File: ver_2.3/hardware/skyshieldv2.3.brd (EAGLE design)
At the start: 17.8 x 43.2 mm, 11 parts, among them J1 HEAD15-NOSS, J2 HEAD15-NOSS-1

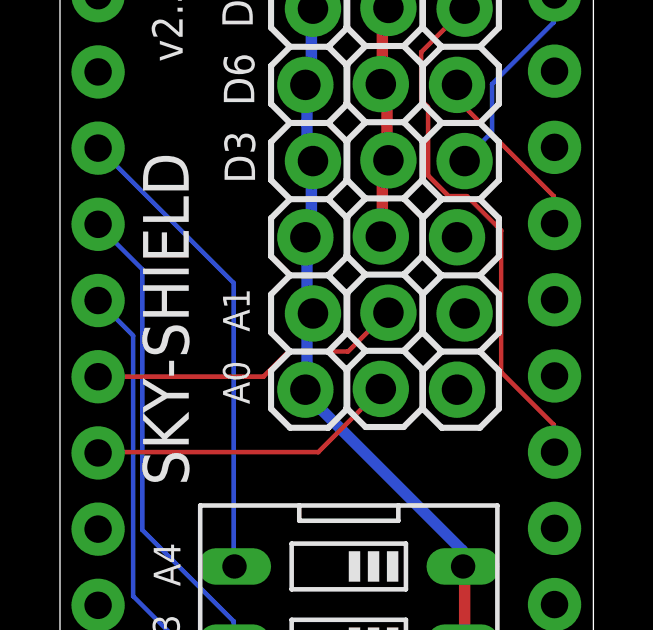
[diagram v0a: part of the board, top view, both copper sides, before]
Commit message: update
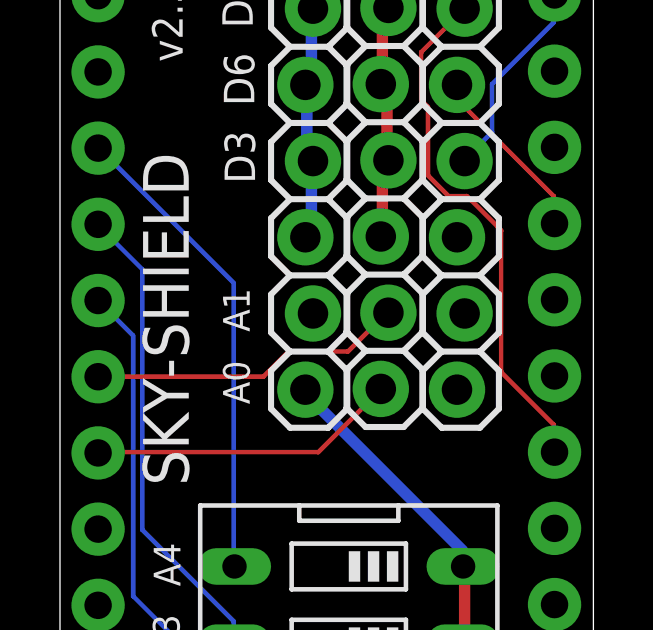
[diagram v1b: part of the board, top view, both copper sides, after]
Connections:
- net GND: no longer JP1.3
- net VCC: no longer JP2.3
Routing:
- net GND: track 65.1 -> 59.4 mm
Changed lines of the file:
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@@
 <contactref element="JP1" pad="5"/>
 <contactref element="JP1" pad="4"/>
-<contactref element="JP1" pad="2"/>
-<contactref element="JP1" pad="1"/>
-<contactref element="JP1" pad="3"/>
 <wire x1="4.953" y1="33.147" x2="6.2484" y2="33.147" width="0.381" layer="16"/>
 <wire x1="1.2954" y1="36.8046" x2="4.953" y2="33.147" width="0.381" layer="16"/>
@@
 <wire x1="13.4874" y1="7.62" x2="13.4366" y2="7.62" width="0.381" layer="1"/>
 <wire x1="13.4874" y1="5.2578" x2="13.4366" y2="5.08" width="0.381" layer="1"/>
-<wire x1="8.2296" y1="15.8496" x2="8.2296" y2="13.5636" width="0.381" layer="16"/>
-<wire x1="8.4328" y1="16.0528" x2="8.2296" y2="15.8496" width="0.381" layer="16"/>
-<wire x1="8.2296" y1="13.5636" x2="8.1788" y2="13.5128" width="0.381" layer="16"/>
-<wire x1="8.2296" y1="16.383" x2="8.2296" y2="18.5928" width="0.381" layer="16"/>
-<wire x1="8.382" y1="16.2306" x2="8.2296" y2="16.383" width="0.381" layer="16"/>
-<wire x1="8.2296" y1="18.5928" x2="8.1788" y2="18.5928" width="0.381" layer="16"/>
-<wire x1="8.382" y1="16.2306" x2="8.4328" y2="16.0528" width="0.381" layer="16"/>
 <wire x1="8.382" y1="18.669" x2="8.382" y2="21.1074" width="0.381" layer="16"/>
 <wire x1="8.382" y1="21.1074" x2="8.4328" y2="21.1328" width="0.381" layer="16"/>
-<wire x1="8.382" y1="18.669" x2="8.1788" y2="18.5928" width="0.381" layer="16"/>
 <wire x1="8.2296" y1="21.1836" x2="8.2296" y2="23.622" width="0.381" layer="16"/>
 <wire x1="8.2296" y1="23.622" x2="8.1788" y2="23.6728" width="0.381" layer="16"/>
@@
 <wire x1="8.2296" y1="13.335" x2="13.4112" y2="8.1534" width="0.381" layer="16"/>
 <wire x1="13.4112" y1="7.62" x2="13.4366" y2="7.62" width="0.381" layer="16"/>
-<wire x1="8.2296" y1="13.335" x2="8.1788" y2="13.5128" width="0.381" layer="16"/>
 <wire x1="6.3246" y1="28.3464" x2="6.3246" y2="32.9184" width="0.381" layer="16"/>
 <wire x1="8.3058" y1="26.3652" x2="6.3246" y2="28.3464" width="0.381" layer="16"/>
 <wire x1="6.3246" y1="32.9184" x2="6.2738" y2="33.0962" width="0.381" layer="16"/>
 <wire x1="8.3058" y1="26.3652" x2="8.4328" y2="26.2128" width="0.381" layer="16"/>
+<contactref element="JP1" pad="1"/>
+<contactref element="JP1" pad="2"/>
+<wire x1="8.4328" y1="16.0528" x2="8.382" y2="18.669" width="0" layer="19" extent="16-16"/>
+<wire x1="8.1788" y1="13.5128" x2="8.4328" y2="16.0528" width="0" layer="19" extent="1-1"/>
+<wire x1="8.2296" y1="13.335" x2="8.1788" y2="13.5128" width="0" layer="19" extent="16-16"/>
 </signal>
 <signal name="VCC" class="1">
@@
 <contactref element="JP2" pad="4"/>
 <contactref element="JP2" pad="5"/>
-<contactref element="JP2" pad="3"/>
 <wire x1="12.954" y1="38.7096" x2="12.954" y2="40.5638" width="0.381" layer="1"/>
 <wire x1="11.3792" y1="37.1348" x2="12.954" y2="38.7096" width="0.381" layer="1"/>
 <wire x1="10.7442" y1="20.955" x2="10.7442" y2="18.669" width="0.381" layer="1"/>
 <wire x1="10.9474" y1="21.1582" x2="10.7442" y2="20.955" width="0.381" layer="1"/>
-<wire x1="10.7442" y1="18.669" x2="10.6934" y2="18.6182" width="0.381" layer="1"/>
 <wire x1="8.0772" y1="29.1084" x2="8.0772" y2="33.0708" width="0.381" layer="1"/>
 <wire x1="10.9474" y1="26.2382" x2="8.0772" y2="29.1084" width="0.381" layer="1"/>
